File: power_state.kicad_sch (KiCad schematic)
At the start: 103 parts, among them Q101 BSZ018N04LS6, Q102 IQE013N04LM6, Q103 BSZ018N04LS6, Q104 IQE013N04LM6, Q105 GS2N7002KW, Q106 GS2N7002KW, U101 UCC27282DRC, U102 ACS37030LLZATR-040B3, U103 UCC27282DRC, U104 ACS37030LLZATR-040B3, U106 INA187A1IDBVR

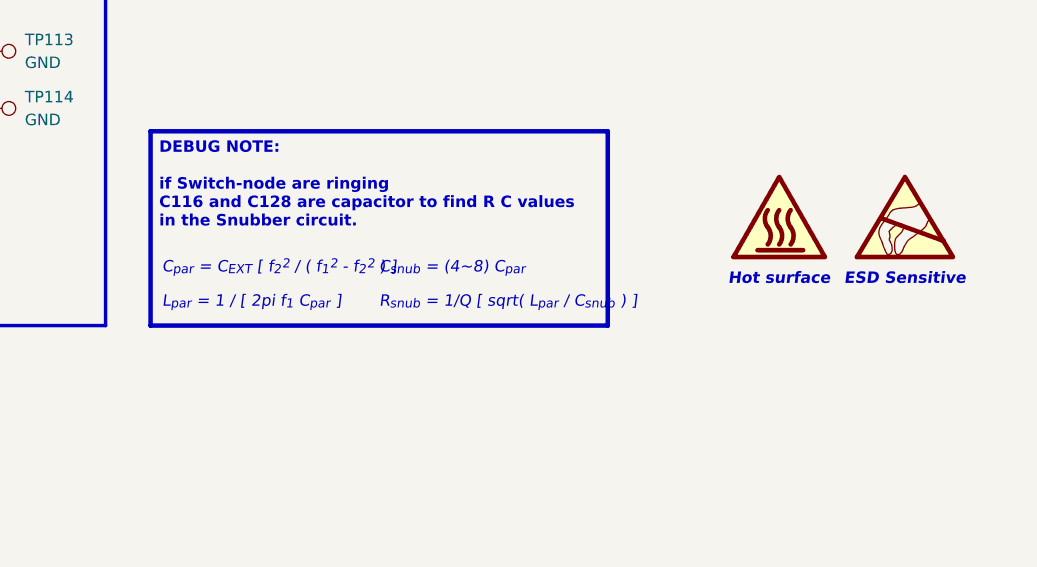
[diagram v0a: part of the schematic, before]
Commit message: Updated Schematic v1.0
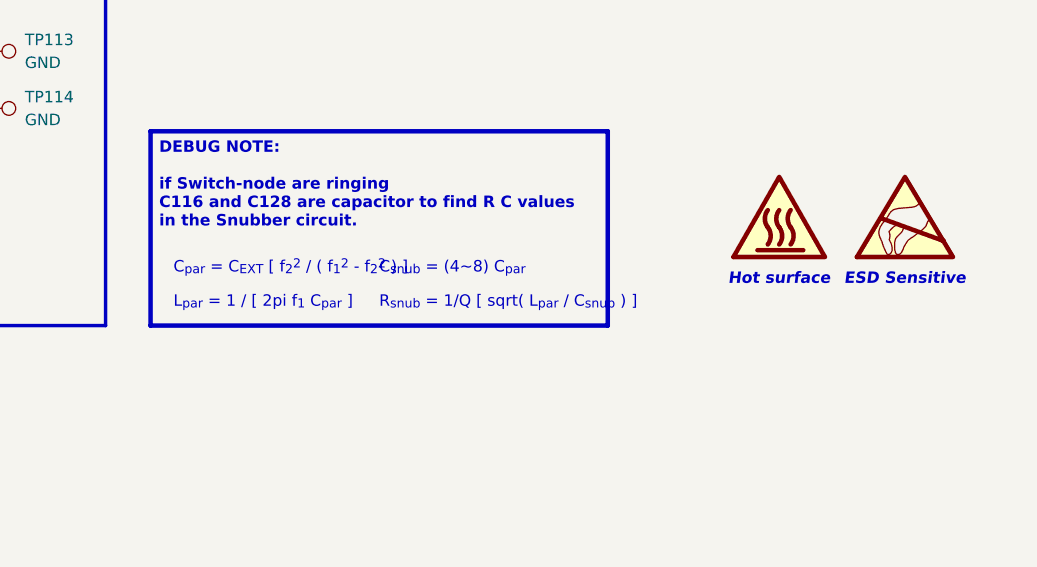
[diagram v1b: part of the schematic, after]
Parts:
- C116, C128: now left out of the parts list
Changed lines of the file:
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@@
 		(effects
 			(font
+				(face "Calibri")
 				(size 1.27 1.27)
-				(italic yes)
 				(color 0 0 0 1)
 			)
@@
 		(effects
 			(font
+				(face "Calibri")
 				(size 1.27 1.27)
-				(italic yes)
 				(color 0 0 0 1)
 			)
@@
 	(text "L_{par} = 1 / [ 2pi f_{1} C_{par} ]"
 		(exclude_from_sim no)
-		(at 165.1 276.86 0)
+		(at 166.37 276.86 0)
 		(effects
 			(font
+				(face "Calibri")
 				(size 1.27 1.27)
-				(italic yes)
 				(color 0 0 0 1)
 			)
@@
 	(text "C_{par} = C_{EXT} [ f_{2}^{2} / ( f_{1}^{2} - f_{2}^{2} ) ]"
 		(exclude_from_sim no)
-		(at 165.1 273.05 0)
+		(at 166.37 273.05 0)
 		(effects
 			(font
+				(face "Calibri")
 				(size 1.27 1.27)
-				(italic yes)
 				(color 0 0 0 1)
 			)
@@
 		(in_bom no)
 		(on_board yes)
-		(in_pos_files yes)
+		(in_pos_files no)
 		(dnp no)
 		(property "Reference" "NT103"
@@
 		(in_bom no)
 		(on_board yes)
-		(in_pos_files yes)
+		(in_pos_files no)
 		(dnp no)
 		(property "Reference" "NT102"
@@
 		(in_bom no)
 		(on_board yes)
-		(in_pos_files yes)
+		(in_pos_files no)
 		(dnp no)
 		(property "Reference" "NT105"
@@
 		(in_bom no)
 		(on_board yes)
-		(in_pos_files yes)
+		(in_pos_files no)
 		(dnp no)
 		(property "Reference" "NT101"
@@
 		(body_style 1)
 		(exclude_from_sim no)
-		(in_bom yes)
+		(in_bom no)
 		(on_board yes)
 		(in_pos_files yes)
@@
 		(body_style 1)
 		(exclude_from_sim no)
-		(in_bom yes)
+		(in_bom no)
 		(on_board yes)
 		(in_pos_files yes)
